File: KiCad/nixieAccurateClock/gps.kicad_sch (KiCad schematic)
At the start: 3 parts

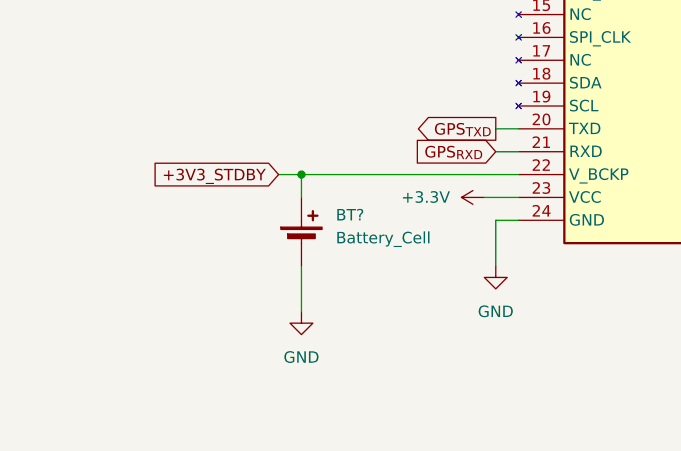
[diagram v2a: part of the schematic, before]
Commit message: Add decoupling caps
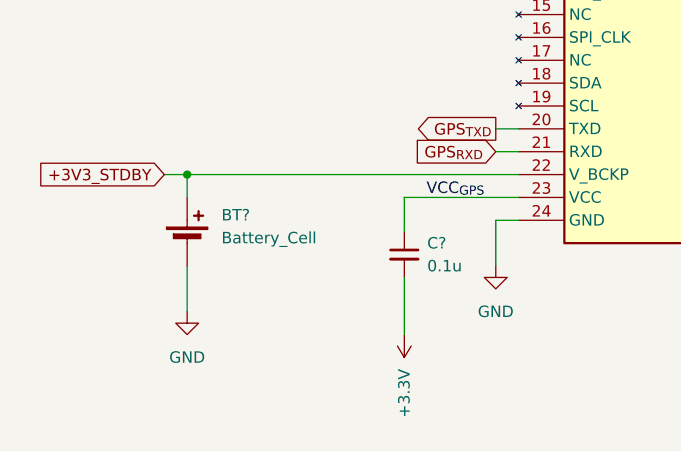
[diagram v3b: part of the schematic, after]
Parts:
- added C?: 0.1u, Capacitor_SMD:C_0603_1608Metric, symbol Device:C_Small
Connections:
- net +3.3V: now also C?.2; no longer U?.23 (VCC)
- new net VCC_{GPS}: C?.1, U?.23 (VCC)
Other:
- moved on the sheet: BT?
